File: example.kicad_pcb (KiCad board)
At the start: 2 copper layers, 40 x 25 mm, 39 parts, among them J1 USB_C_Receptacle_USB2.0_16P, J2 SSD1309 24-Pin Connector, J3 SSD1327 16-Pin Connector, J4 SSD1322 30-Pin Connector, U1 AP2112K-3.3, U2 ESP32-S3-WROOM-1, U3 MT3608

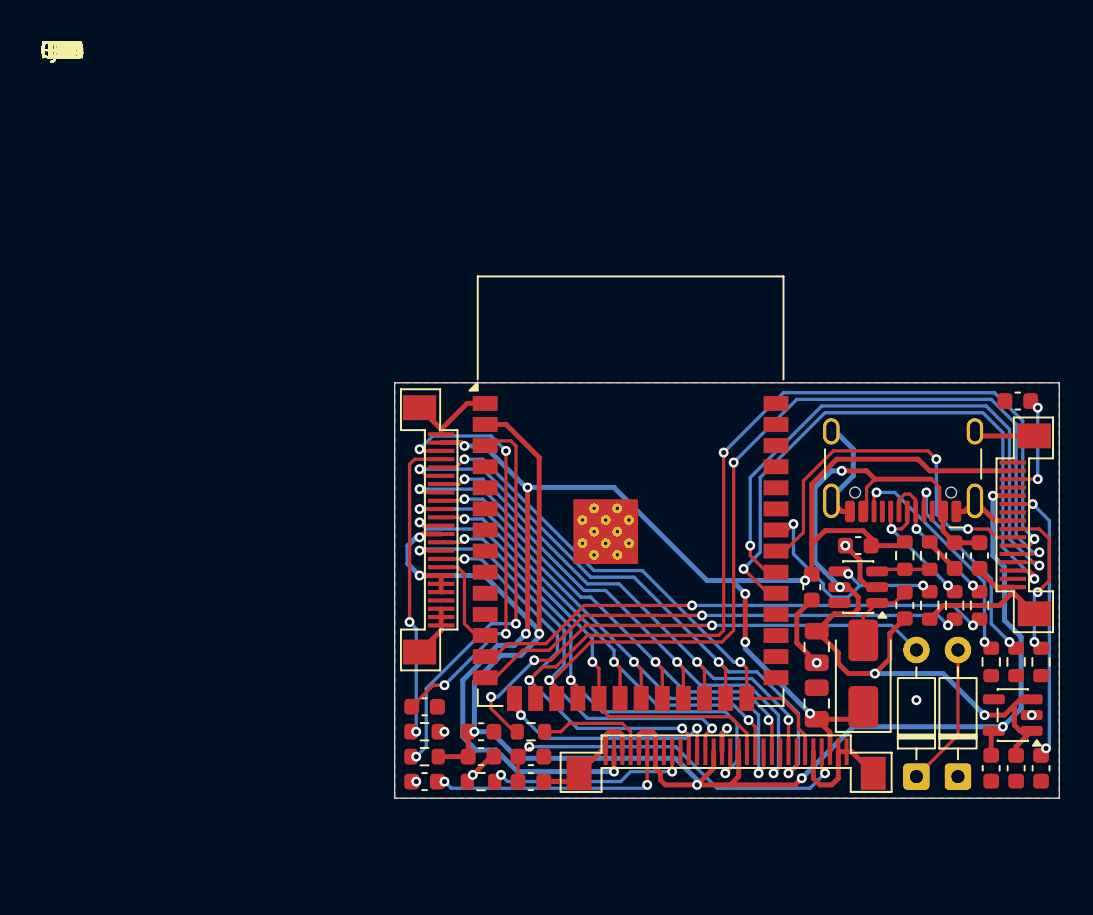
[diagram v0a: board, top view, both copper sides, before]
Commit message: PCB layout part 3
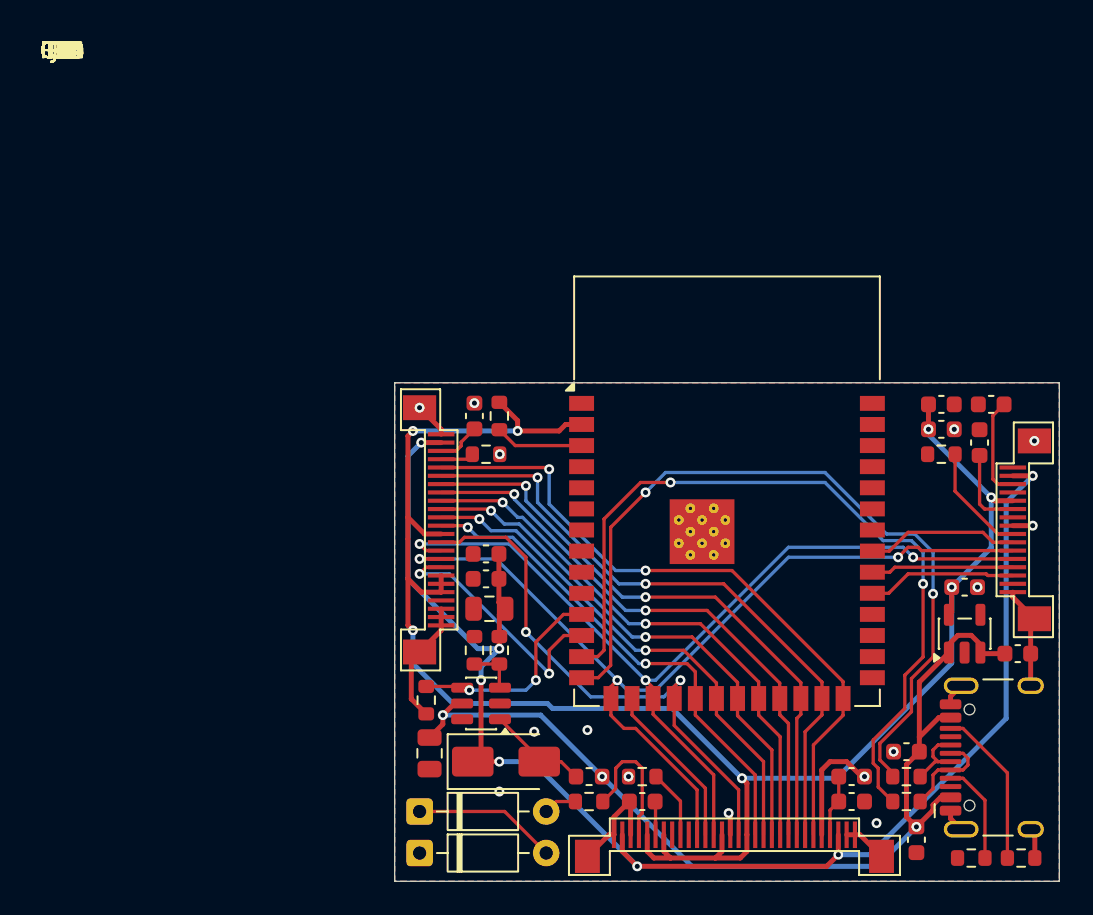
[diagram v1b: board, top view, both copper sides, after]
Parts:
- moved C7 34.0 mm to (52.9, 22.8)
- moved C9 34.0 mm to (52.9, 21.3)
- moved D2 32.7 mm to (21.5, 48.3), turned to 0 degrees
- moved R10 30.8 mm to (21.9, 39.1)
- moved D1 30.0 mm to (21.5, 45.8), turned to 0 degrees
- moved R12 28.0 mm to (24.8, 36.1)
- moved R11 25.1 mm to (26.3, 36.1)
- moved C13 24.2 mm to (22.1, 42.3)
- moved U3 23.8 mm to (25.2, 39.3)
- moved C16 22.4 mm to (25.5, 30.3)
- moved D3 22.1 mm to (26.7, 42.8), turned to 0 degrees
- moved L1 21.6 mm to (31.7, 43.7), turned to 180 degrees
- moved R7 21.0 mm to (26.3, 22.0), turned to -90 degrees
- moved C14 20.5 mm to (25.7, 33.6), turned to 180 degrees
- moved C6 19.9 mm to (55.2, 23.6), turned to 90 degrees
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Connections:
- U2 pad 11: unconnected-(U2-IO18-Pad11) -> /MT3608/EN
- U2 pad 15: /CS_1322 -> /RES
- U2 pad 16: /RES -> /CS_1322
- U2 pad 34: /MT3608/EN -> unconnected-(U2-IO41-Pad34)
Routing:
- net Net-(D1-A): track 30.8 -> 2.00 mm, vias 3 -> 0
- net /MOSI: track 36.5 -> 8.98 mm, vias 2 -> 0
- net /CLK: track 35.4 -> 8.57 mm, vias 2 -> 0
- net /DC: track 81.3 -> 55.2 mm, vias 5 -> 3
- net GND: track 62.6 -> 39.2 mm, vias 8 -> 15
- net Net-(J2-VCOMH): track 25.7 -> 2.68 mm, vias 4 -> 0
- net /RES: track 78.3 -> 55.9 mm, vias 5 -> 3
- net Net-(J4-VCOMH): track 23.0 -> 3.72 mm, vias 2 -> 0
- net Net-(U2-EN): track 24.5 -> 5.35 mm, vias 2 -> 0
- net Net-(U2-USB_D+): track 30.5 -> 48.3 mm
- net Net-(J2-IREF): track 18.6 -> 2.00 mm, vias 2 -> 0
- net Net-(U2-USB_D-): track 31.7 -> 48.0 mm
- net /CS_1327: track 22.7 -> 9.17 mm, vias 2 -> 0
- net Net-(J4-VDD): track 14.4 -> 2.01 mm, vias 2 -> 0
- net Net-(J3-VDD): track 16.9 -> 5.05 mm, vias 2 -> 0
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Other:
- board size 40 x 25 mm -> 40 x 30 mm
